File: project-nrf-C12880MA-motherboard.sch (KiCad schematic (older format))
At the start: 22 parts, among them J1 Left, J2 Right, J3 PJ-036AH-SMT-TR, J4 SM04B-SRSS-TB(LF)(SN), J5 SM04B-SRSS-TB(LF)(SN), J6 SM04B-SRSS-TB(LF)(SN), J7 1702473, J8 C12880MA Breakboard v2, U1 ADS1219IPWR, U2 TPS7A0350PDBVR, U3 LSF0204DPWR

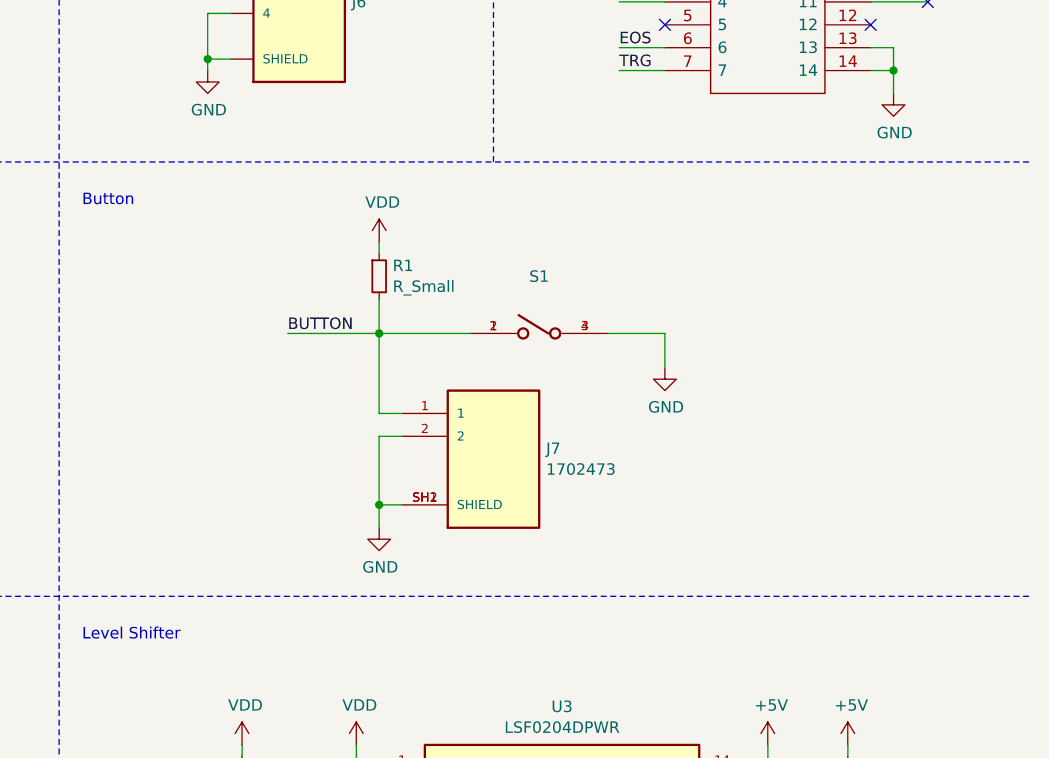
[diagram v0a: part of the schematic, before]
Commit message: First placement
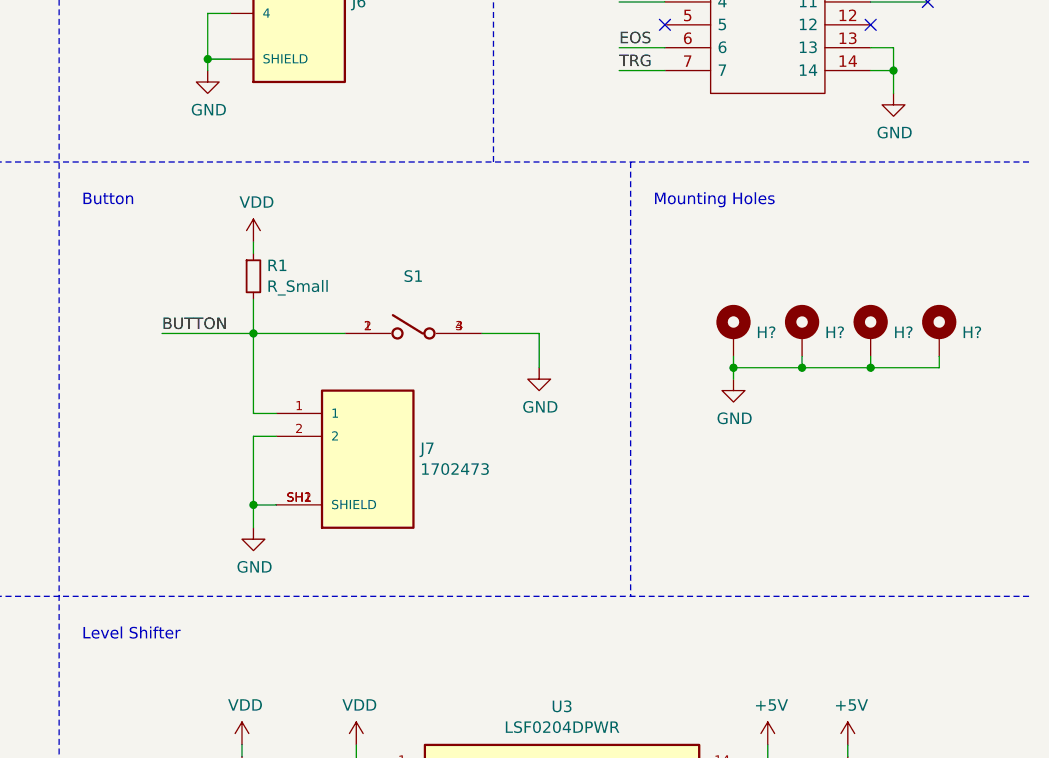
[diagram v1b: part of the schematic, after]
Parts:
- added H? (x4): MountingHole_Pad, MountingHole:MountingHole_2.7mm_M2.5_Pad_Via, symbol Mechanical:MountingHole_Pad
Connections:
- net GND: now also H?.1, H?.1, H?.1, H?.1
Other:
- note added: "Mounting Holes"
- moved on the sheet: J7, R1, S1
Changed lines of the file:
@@
 L power:GND #PWR0104
 U 1 1 6234D28E
-P 9600 2950
-F 0 "#PWR0104" H 9600 2700 50  0001 C CNN
-F 1 "GND" H 9605 2777 50  0000 C CNN
-F 2 "" H 9600 2950 50  0001 C CNN
-F 3 "" H 9600 2950 50  0001 C CNN
-	1    9600 2950
-	1    0    0    -1
-$EndComp
-Text Label 7950 2800 0    50   ~ 0
+P 9050 2950
+F 0 "#PWR0104" H 9050 2700 50  0001 C CNN
+F 1 "GND" H 9055 2777 50  0000 C CNN
+F 2 "" H 9050 2950 50  0001 C CNN
+F 3 "" H 9050 2950 50  0001 C CNN
+	1    9050 2950
+	1    0    0    -1
+$EndComp
+Text Label 7400 2800 0    50   ~ 0
 BUTTON
 $Comp
 L Device:R_Small R1
 U 1 1 62359C57
-P 8350 2550
-F 0 "R1" H 8409 2596 50  0000 L CNN
-F 1 "R_Small" H 8409 2505 50  0000 L CNN
-F 2 "Resistor_SMD:R_0603_1608Metric" H 8350 2550 50  0001 C CNN
-F 3 "~" H 8350 2550 50  0001 C CNN
-	1    8350 2550
+P 7800 2550
+F 0 "R1" H 7859 2596 50  0000 L CNN
+F 1 "R_Small" H 7859 2505 50  0000 L CNN
+F 2 "Resistor_SMD:R_0603_1608Metric" H 7800 2550 50  0001 C CNN
+F 3 "~" H 7800 2550 50  0001 C CNN
+	1    7800 2550
 	1    0    0    -1
 $EndComp
@@
 L B3FS-1010P:B3FS-1010P S1
 U 1 1 6236F713
-P 9050 2800
-F 0 "S1" H 9050 3049 50  0000 C CNN
-F 1 "B3FS-1010P" H 9050 2958 50  0001 C CNN
-F 2 "B3FS-1010:SW_B3FS-1010P" H 9050 2800 50  0001 L BNN
-F 3 "" H 9050 2800 50  0001 L BNN
-F 4 "Compliant" H 9050 2800 50  0001 L BNN "EU_RoHS_Compliance"
-F 5 "B3FS-1010P" H 9050 2800 50  0001 L BNN "Comment"
-	1    9050 2800
-	1    0    0    -1
-$EndComp
-Wire Wire Line
-	9350 2800 9600 2800
-Wire Wire Line
-	7950 2800 8350 2800
-Wire Wire Line
-	8350 2650 8350 2800
-Connection ~ 8350 2800
-Wire Wire Line
-	8350 2800 8750 2800
-Wire Wire Line
-	9600 2800 9600 2950
+P 8500 2800
+F 0 "S1" H 8500 3049 50  0000 C CNN
+F 1 "B3FS-1010P" H 8500 2958 50  0001 C CNN
+F 2 "B3FS-1010:SW_B3FS-1010P" H 8500 2800 50  0001 L BNN
+F 3 "" H 8500 2800 50  0001 L BNN
+F 4 "Compliant" H 8500 2800 50  0001 L BNN "EU_RoHS_Compliance"
+F 5 "B3FS-1010P" H 8500 2800 50  0001 L BNN "Comment"
+	1    8500 2800
+	1    0    0    -1
+$EndComp
+Wire Wire Line
+	8800 2800 9050 2800
+Wire Wire Line
+	7400 2800 7800 2800
+Wire Wire Line
+	7800 2650 7800 2800
+Connection ~ 7800 2800
+Wire Wire Line
+	7800 2800 8200 2800
+Wire Wire Line
+	9050 2800 9050 2950
 $Comp
 L power:+5V #PWR010
@@
 $EndComp
 Wire Wire Line
-	8350 2400 8350 2450
+	7800 2400 7800 2450
 $Comp
 L TPS7A0233PDBVR:TPS7A0233PDBVR U2
@@
 L power:VDD #PWR027
 U 1 1 6257331C
-P 8350 2400
-F 0 "#PWR027" H 8350 2250 50  0001 C CNN
-F 1 "VDD" H 8365 2573 50  0000 C CNN
-F 2 "" H 8350 2400 50  0001 C CNN
-F 3 "" H 8350 2400 50  0001 C CNN
-	1    8350 2400
+P 7800 2400
+F 0 "#PWR027" H 7800 2250 50  0001 C CNN
+F 1 "VDD" H 7815 2573 50  0000 C CNN
+F 2 "" H 7800 2400 50  0001 C CNN
+F 3 "" H 7800 2400 50  0001 C CNN
+	1    7800 2400
 	1    0    0    -1
 $EndComp
@@
 L 1702473:1702473 J7
 U 1 1 62584EF1
-P 8850 3350
-F 0 "J7" H 9080 3396 50  0000 L CNN
-F 1 "1702473" H 9080 3305 50  0000 L CNN
-F 2 "PHOENIX_1702473" H 8850 3350 50  0001 L BNN
-F 3 "" H 8850 3350 50  0001 L BNN
-F 4 "Manufacturer Recommendations" H 8850 3350 50  0001 L BNN "STANDARD"
-F 5 "Phoenix Contact" H 8850 3350 50  0001 L BNN "MANUFACTURER"
-F 6 "MAR20,2012" H 8850 3350 50  0001 L BNN "PARTREV"
-	1    8850 3350
+P 8300 3350
+F 0 "J7" H 8530 3396 50  0000 L CNN
+F 1 "1702473" H 8530 3305 50  0000 L CNN
+F 2 "PHOENIX_1702473" H 8300 3350 50  0001 L BNN
+F 3 "" H 8300 3350 50  0001 L BNN
+F 4 "Manufacturer Recommendations" H 8300 3350 50  0001 L BNN "STANDARD"
+F 5 "Phoenix Contact" H 8300 3350 50  0001 L BNN "MANUFACTURER"
+F 6 "MAR20,2012" H 8300 3350 50  0001 L BNN "PARTREV"
+	1    8300 3350
 	1    0    0    -1
 $EndComp
@@
 $EndComp
 Wire Wire Line
-	8450 3150 8350 3150
-Wire Wire Line
-	8350 3150 8350 2800
+	7900 3150 7800 3150
+Wire Wire Line
+	7800 3150 7800 2800
 $Comp
 L power:GND #PWR028
 U 1 1 625F1955
-P 8350 3650
-F 0 "#PWR028" H 8350 3400 50  0001 C CNN
-F 1 "GND" H 8355 3477 50  0000 C CNN
-F 2 "" H 8350 3650 50  0001 C CNN
-F 3 "" H 8350 3650 50  0001 C CNN
-	1    8350 3650
-	1    0    0    -1
-$EndComp
-Wire Wire Line
-	8450 3550 8350 3550
-Wire Wire Line
-	8350 3550 8350 3650
-Wire Wire Line
-	8450 3250 8350 3250
-Wire Wire Line
-	8350 3250 8350 3550
-Connection ~ 8350 3550
+P 7800 3650
+F 0 "#PWR028" H 7800 3400 50  0001 C CNN
+F 1 "GND" H 7805 3477 50  0000 C CNN
+F 2 "" H 7800 3650 50  0001 C CNN
+F 3 "" H 7800 3650 50  0001 C CNN
+	1    7800 3650
+	1    0    0    -1
+$EndComp
+Wire Wire Line
+	7900 3550 7800 3550
+Wire Wire Line
+	7800 3550 7800 3650
+Wire Wire Line
+	7900 3250 7800 3250
+Wire Wire Line
+	7800 3250 7800 3550
+Connection ~ 7800 3550
 $Comp
 L Device:C_Small C6
@@
 NoConn ~ 1100 2950
 Wire Notes Line
-	500  2050 11200 2050
-Wire Notes Line
 	500  3950 11200 3950
 Wire Notes Line
@@
 Text Label 1250 5450 0    50   ~ 0
 VIDEO
+$Comp
+L Mechanical:MountingHole_Pad H?
+U 1 1 62DE7F5A
+P 10800 2800
+F 0 "H?" H 10900 2803 50  0000 L CNN
+F 1 "MountingHole_Pad" H 10900 2758 50  0001 L CNN
+F 2 "MountingHole:MountingHole_2.7mm_M2.5_Pad_Via" H 10800 2800 50  0001 C CNN
+F 3 "~" H 10800 2800 50  0001 C CNN
+	1    10800 2800
+	1    0    0    -1
+$EndComp
+$Comp
+L Mechanical:MountingHole_Pad H?
+U 1 1 62DE790A
+P 10500 2800
+F 0 "H?" H 10600 2803 50  0000 L CNN
+F 1 "MountingHole_Pad" H 10600 2758 50  0001 L CNN
+F 2 "MountingHole:MountingHole_2.7mm_M2.5_Pad_Via" H 10500 2800 50  0001 C CNN
+F 3 "~" H 10500 2800 50  0001 C CNN
+	1    10500 2800
+	1    0    0    -1
+$EndComp
+$Comp
+L Mechanical:MountingHole_Pad H?
+U 1 1 62DE712E
+P 10200 2800
+F 0 "H?" H 10300 2803 50  0000 L CNN
+F 1 "MountingHole_Pad" H 10300 2758 50  0001 L CNN
+F 2 "MountingHole:MountingHole_2.7mm_M2.5_Pad_Via" H 10200 2800 50  0001 C CNN
+F 3 "~" H 10200 2800 50  0001 C CNN
+	1    10200 2800
+	1    0    0    -1
+$EndComp
+$Comp
+L Mechanical:MountingHole_Pad H?
+U 1 1 62DE5DC9
+P 9900 2800
+F 0 "H?" H 10000 2803 50  0000 L CNN
+F 1 "MountingHole_Pad" H 10000 2758 50  0001 L CNN
+F 2 "MountingHole:MountingHole_2.7mm_M2.5_Pad_Via" H 9900 2800 50  0001 C CNN
+F 3 "~" H 9900 2800 50  0001 C CNN
+	1    9900 2800
+	1    0    0    -1
+$EndComp
+$Comp
+L power:GND #PWR?
+U 1 1 62DF80EC
+P 9900 3000
+F 0 "#PWR?" H 9900 2750 50  0001 C CNN
+F 1 "GND" H 9905 2827 50  0000 C CNN
+F 2 "" H 9900 3000 50  0001 C CNN
+F 3 "" H 9900 3000 50  0001 C CNN
+	1    9900 3000
+	1    0    0    -1
+$EndComp
+Wire Wire Line
+	9900 2900 9900 2950
+Wire Wire Line
+	9900 2950 10200 2950
+Wire Wire Line
+	10200 2950 10200 2900
+Connection ~ 9900 2950
+Wire Wire Line
+	9900 2950 9900 3000
+Wire Wire Line
+	10500 2900 10500 2950
+Wire Wire Line
+	10500 2950 10200 2950
+Connection ~ 10200 2950
+Wire Wire Line
+	10800 2900 10800 2950
+Wire Wire Line
+	10800 2950 10500 2950
+Connection ~ 10500 2950
+Wire Notes Line
+	500  2050 11200 2050
+Wire Notes Line
+	9450 2050 9450 3950
+Text Notes 9550 2250 0    50   ~ 0
+Mounting Holes
 $EndSCHEMATC

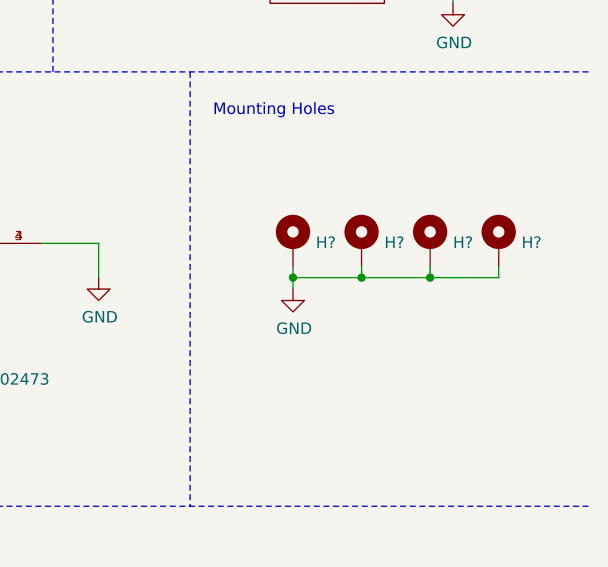
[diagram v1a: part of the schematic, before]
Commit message: Placement 2
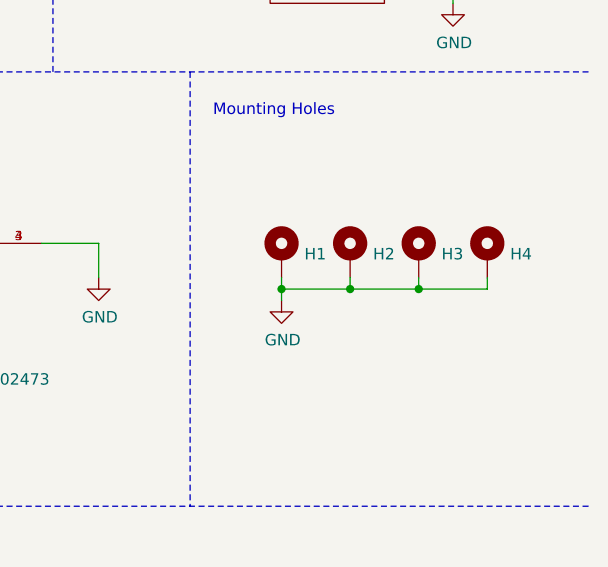
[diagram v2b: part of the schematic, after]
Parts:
- gave numbers to parts that had none: 4
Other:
- moved on the sheet: H1, H2, H3, H4
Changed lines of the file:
@@
 VIDEO
 $Comp
-L Mechanical:MountingHole_Pad H?
+L Mechanical:MountingHole_Pad H4
 U 1 1 62DE7F5A
-P 10800 2800
-F 0 "H?" H 10900 2803 50  0000 L CNN
-F 1 "MountingHole_Pad" H 10900 2758 50  0001 L CNN
-F 2 "MountingHole:MountingHole_2.7mm_M2.5_Pad_Via" H 10800 2800 50  0001 C CNN
-F 3 "~" H 10800 2800 50  0001 C CNN
-	1    10800 2800
+P 10750 2850
+F 0 "H4" H 10850 2853 50  0000 L CNN
+F 1 "MountingHole_Pad" H 10850 2808 50  0001 L CNN
+F 2 "MountingHole:MountingHole_2.7mm_M2.5_Pad_Via" H 10750 2850 50  0001 C CNN
+F 3 "~" H 10750 2850 50  0001 C CNN
+	1    10750 2850
 	1    0    0    -1
 $EndComp
 $Comp
-L Mechanical:MountingHole_Pad H?
+L Mechanical:MountingHole_Pad H3
 U 1 1 62DE790A
-P 10500 2800
-F 0 "H?" H 10600 2803 50  0000 L CNN
-F 1 "MountingHole_Pad" H 10600 2758 50  0001 L CNN
-F 2 "MountingHole:MountingHole_2.7mm_M2.5_Pad_Via" H 10500 2800 50  0001 C CNN
-F 3 "~" H 10500 2800 50  0001 C CNN
-	1    10500 2800
+P 10450 2850
+F 0 "H3" H 10550 2853 50  0000 L CNN
+F 1 "MountingHole_Pad" H 10550 2808 50  0001 L CNN
+F 2 "MountingHole:MountingHole_2.7mm_M2.5_Pad_Via" H 10450 2850 50  0001 C CNN
+F 3 "~" H 10450 2850 50  0001 C CNN
+	1    10450 2850
 	1    0    0    -1
 $EndComp
 $Comp
-L Mechanical:MountingHole_Pad H?
+L Mechanical:MountingHole_Pad H2
 U 1 1 62DE712E
-P 10200 2800
-F 0 "H?" H 10300 2803 50  0000 L CNN
-F 1 "MountingHole_Pad" H 10300 2758 50  0001 L CNN
-F 2 "MountingHole:MountingHole_2.7mm_M2.5_Pad_Via" H 10200 2800 50  0001 C CNN
-F 3 "~" H 10200 2800 50  0001 C CNN
-	1    10200 2800
+P 10150 2850
+F 0 "H2" H 10250 2853 50  0000 L CNN
+F 1 "MountingHole_Pad" H 10250 2808 50  0001 L CNN
+F 2 "MountingHole:MountingHole_2.7mm_M2.5_Pad_Via" H 10150 2850 50  0001 C CNN
+F 3 "~" H 10150 2850 50  0001 C CNN
+	1    10150 2850
 	1    0    0    -1
 $EndComp
 $Comp
-L Mechanical:MountingHole_Pad H?
+L Mechanical:MountingHole_Pad H1
 U 1 1 62DE5DC9
-P 9900 2800
-F 0 "H?" H 10000 2803 50  0000 L CNN
-F 1 "MountingHole_Pad" H 10000 2758 50  0001 L CNN
-F 2 "MountingHole:MountingHole_2.7mm_M2.5_Pad_Via" H 9900 2800 50  0001 C CNN
-F 3 "~" H 9900 2800 50  0001 C CNN
-	1    9900 2800
+P 9850 2850
+F 0 "H1" H 9950 2853 50  0000 L CNN
+F 1 "MountingHole_Pad" H 9950 2808 50  0001 L CNN
+F 2 "MountingHole:MountingHole_2.7mm_M2.5_Pad_Via" H 9850 2850 50  0001 C CNN
+F 3 "~" H 9850 2850 50  0001 C CNN
+	1    9850 2850
 	1    0    0    -1
 $EndComp
 $Comp
-L power:GND #PWR?
+L power:GND #PWR035
 U 1 1 62DF80EC
-P 9900 3000
-F 0 "#PWR?" H 9900 2750 50  0001 C CNN
-F 1 "GND" H 9905 2827 50  0000 C CNN
-F 2 "" H 9900 3000 50  0001 C CNN
-F 3 "" H 9900 3000 50  0001 C CNN
-	1    9900 3000
+P 9850 3050
+F 0 "#PWR035" H 9850 2800 50  0001 C CNN
+F 1 "GND" H 9855 2877 50  0000 C CNN
+F 2 "" H 9850 3050 50  0001 C CNN
+F 3 "" H 9850 3050 50  0001 C CNN
+	1    9850 3050
 	1    0    0    -1
 $EndComp
 Wire Wire Line
-	9900 2900 9900 2950
+	9850 2950 9850 3000
 Wire Wire Line
-	9900 2950 10200 2950
+	9850 3000 10150 3000
 Wire Wire Line
-	10200 2950 10200 2900
-Connection ~ 9900 2950
+	10150 3000 10150 2950
+Connection ~ 9850 3000
 Wire Wire Line
-	9900 2950 9900 3000
+	9850 3000 9850 3050
 Wire Wire Line
-	10500 2900 10500 2950
+	10450 2950 10450 3000
 Wire Wire Line
-	10500 2950 10200 2950
-Connection ~ 10200 2950
+	10450 3000 10150 3000
+Connection ~ 10150 3000
 Wire Wire Line
-	10800 2900 10800 2950
+	10750 2950 10750 3000
 Wire Wire Line
-	10800 2950 10500 2950
-Connection ~ 10500 2950
+	10750 3000 10450 3000
+Connection ~ 10450 3000
 Wire Notes Line
 	500  2050 11200 2050
